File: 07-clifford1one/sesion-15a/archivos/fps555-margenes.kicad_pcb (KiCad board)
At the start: 2 copper layers, 100 x 50 mm, 23 parts, among them J1 Batería 9v, M1 Motorreductor, U1 555, U2 L293D, U3 mst303

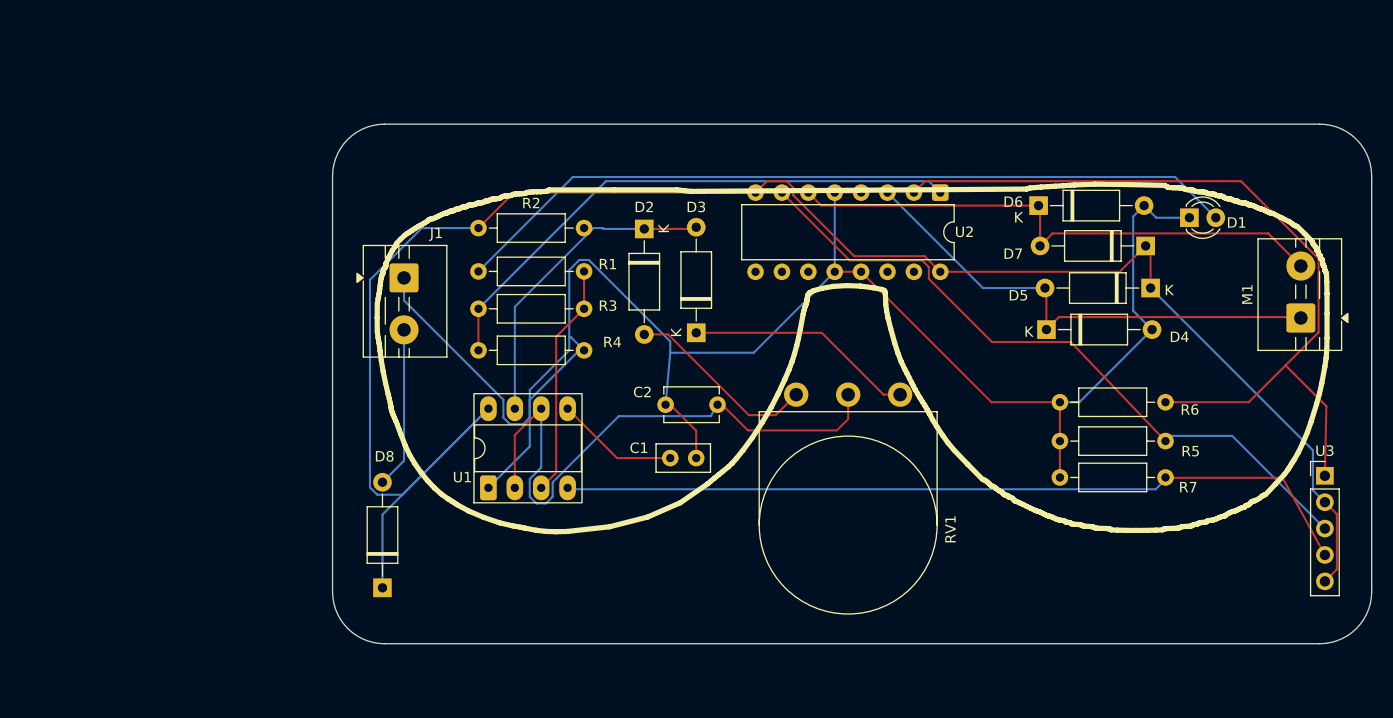
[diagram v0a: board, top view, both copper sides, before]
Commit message: pcb
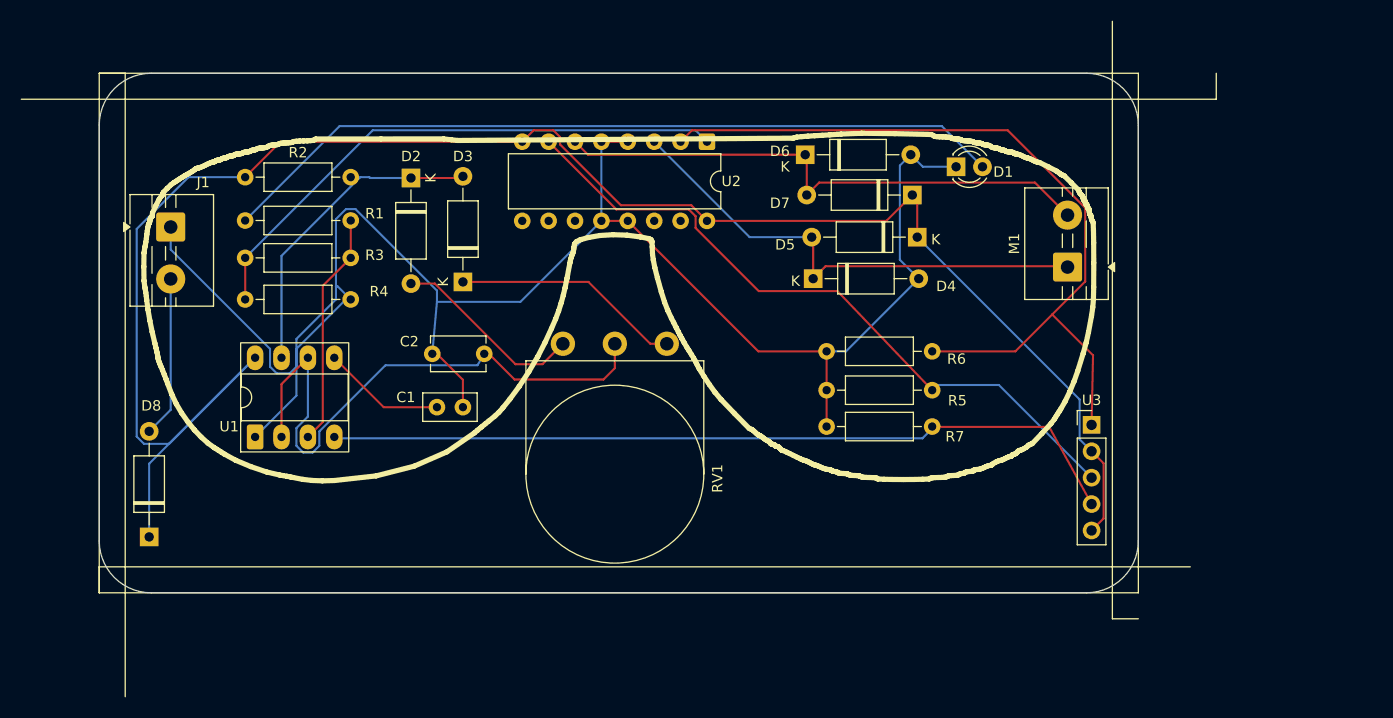
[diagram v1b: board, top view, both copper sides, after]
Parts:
- moved D1 23.0 mm to (112.5, 54.0)
- moved C1 23.0 mm to (62.5, 77.1)
- moved C2 23.0 mm to (67.0, 72.0)
- moved D2 23.0 mm to (60.0, 55.1)
- moved D3 23.0 mm to (65.0, 65.1)
- moved D5 23.0 mm to (108.7, 60.8)
- moved D6 23.0 mm to (97.9, 52.8)
- moved M1 23.0 mm to (123.2, 63.7)
- moved R5 23.0 mm to (100.0, 75.5)
- moved R7 23.0 mm to (100.0, 79.0)
- moved U1 23.0 mm to (45.0, 80.0)
- moved U2 23.0 mm to (88.5, 51.6)
- moved U3 23.0 mm to (125.5, 78.8)
- moved D4 23.0 mm to (98.7, 64.8)
- moved R6 23.0 mm to (100.0, 71.8)
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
